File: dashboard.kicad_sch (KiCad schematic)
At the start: 30 parts, among them J1 DT13-12PA-B016, J3 RJ45, J5 776267-1, Q1 2N7002, SW1 SW_Push, SW2 SW_SPST, SW4 SW_SPST, U1 TPS542025DDC, U4 ILD74

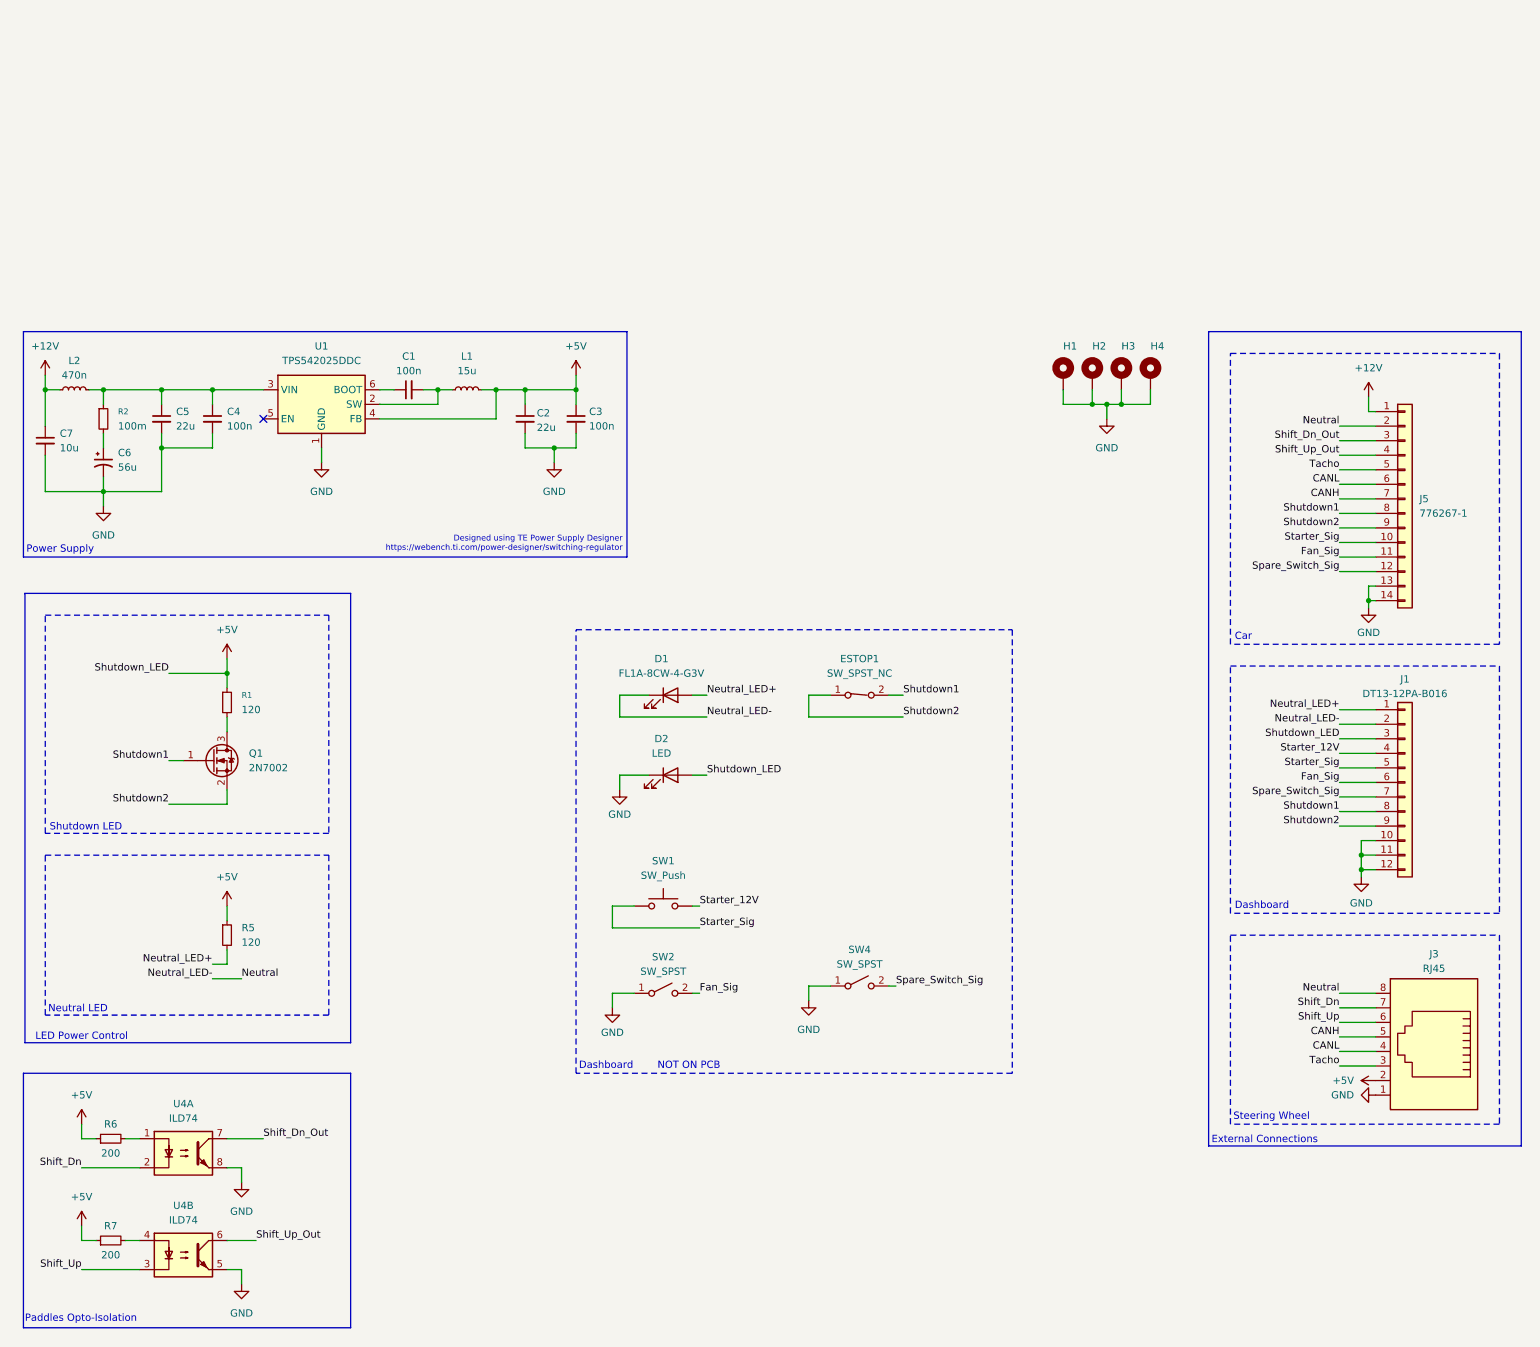
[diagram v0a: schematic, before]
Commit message: Route PCB
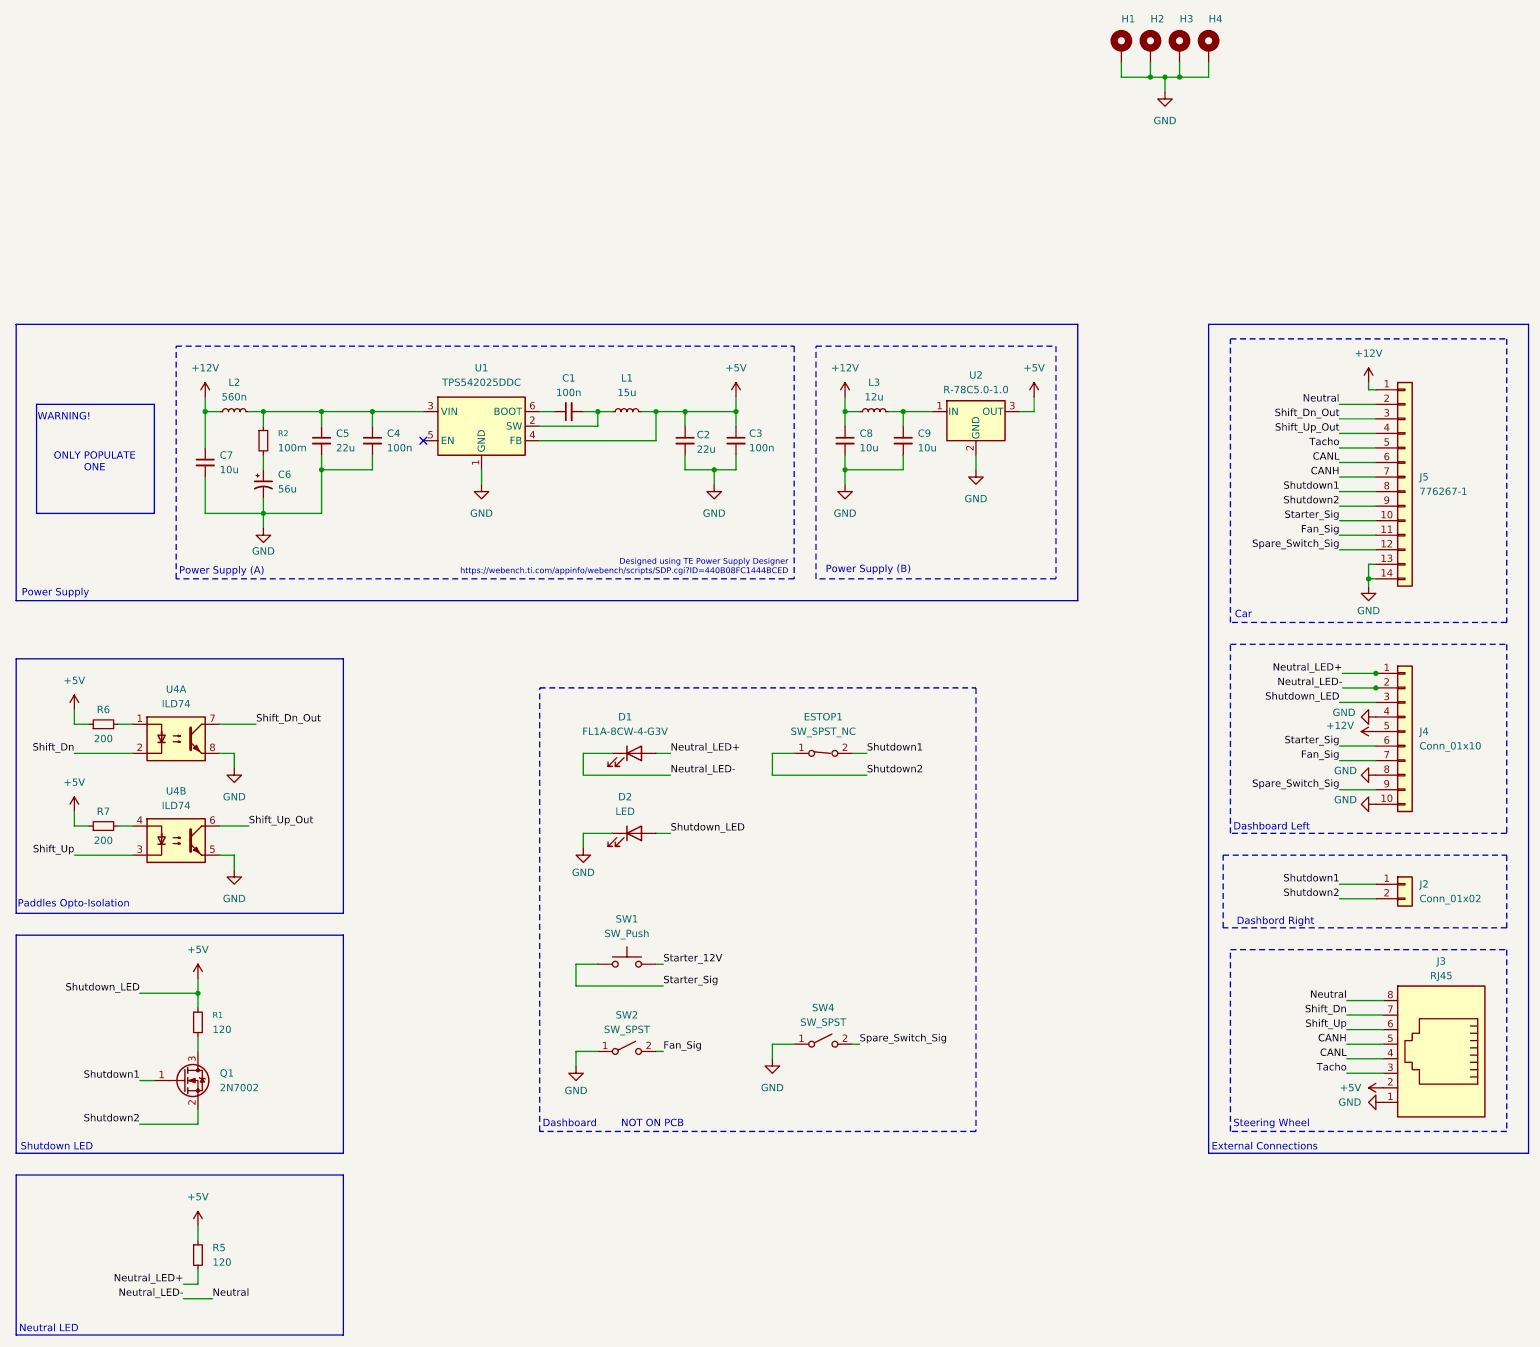
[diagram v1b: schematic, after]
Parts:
- removed J1: DT13-12PA-B016, symbol Connector_Generic:Conn_01x12
- added C8, C9: 10u, Capacitor_THT:C_Disc_D5.1mm_W3.2mm_P5.00mm, symbol Device:C_Small
- added J2: Conn_01x02, Connector_JST:JST_EH_B2B-EH-A_1x02_P2.50mm_Vertical, symbol Connector_Generic:Conn_01x02
- added J4: Conn_01x10, Connector_JST:JST_EH_B10B-EH-A_1x10_P2.50mm_Vertical, symbol Connector_Generic:Conn_01x10
- added L3: 12u, Inductor_SMD:L_Wuerth_WE-PD-Typ-7345, symbol Device:L_Small
- added U2: R-78C5.0-1.0, Converter_DCDC:Converter_DCDC_RECOM_R-78E-0.5_THT, symbol Regulator_Switching:R-78C5.0-1.0
- C1, C2, C3, C4: footprint (none) -> Capacitor_SMD:C_0805_2012Metric_Pad1.18x1.45mm_HandSolder; now left out of the parts list
- C5, C7: footprint (none) -> Capacitor_SMD:C_1210_3225Metric_Pad1.33x2.70mm_HandSolder; now left out of the parts list
- C6: footprint (none) -> Capacitor_SMD:C_Elec_6.3x5.8; now left out of the parts list
- D2, ESTOP1, SW4, U1: now left out of the parts list
- L1: footprint (none) -> Inductor_SMD:L_TDK_SLF12575; now left out of the parts list
- L2: value 470n -> 560n; footprint (none) -> Inductor_SMD:L_Wuerth_MAPI-3012; now left out of the parts list
- Q1: footprint Package_TO_SOT_SMD:SOT-23 -> Package_TO_SOT_THT:TO-92L_Inline_Wide
- R1: footprint (none) -> Resistor_THT:R_Axial_DIN0207_L6.3mm_D2.5mm_P7.62mm_Horizontal
- R2: footprint (none) -> Resistor_SMD:R_0805_2012Metric_Pad1.20x1.40mm_HandSolder; now left out of the parts list
- R6, R7: footprint Resistor_SMD:R_0603_1608Metric_Pad0.98x0.95mm_HandSolder -> Resistor_THT:R_Axial_DIN0207_L6.3mm_D2.5mm_P7.62mm_Horizontal
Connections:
- net +12V: now also C8.1, J4.5 (Pin_5), L3.1
- net +5V: now also J4.3 (Pin_3), U2.3 (OUT)
- net Fan_Sig: now also J4.7 (Pin_7)
- net GND: now also C8.2, C9.2, J4.10 (Pin_10), J4.4 (Pin_4), J4.8 (Pin_8), U2.2 (GND)
- net Neutral: now also J4.2 (Pin_2)
- net Neutral_LED+: now also J4.1 (Pin_1)
- net Shutdown1: now also J2.1 (Pin_1)
- net Shutdown2: now also J2.2 (Pin_2)
- net Spare_Switch_Sig: now also J4.9 (Pin_9)
- net Starter_Sig: now also J4.6 (Pin_6)
- new net: C9.1, L3.2, U2.1 (IN)
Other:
- note added: "Dashboard Left"
- note added: "Dashbord Right"
- note added: "Designed using TE Power Supply Designer https://webench.ti.com/appinfo/webench/scripts/SDP.cgi?ID=440B08FC1444BCED"
- note added: "ONLY POPULATE ONE"
- note added: "Power Supply (A)"
- note added: "Power Supply (B)"
- note added: "WARNING!"
- note removed: "Designed using TE Power Supply Designer https://webench.ti.com/power-designer/switching-regulator"
- note removed: "LED Power Control"
- moved on the sheet: C1, C2, C3, C4, C5, C6, C7, D1, D2, ESTOP1, H1, H2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
